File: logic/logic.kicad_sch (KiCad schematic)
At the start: 32 parts, among them J1 DIN41612_03x32_ABC, J2 Conn_02x05_Odd_Even, J3 Conn_02x05_Odd_Even, J5 Conn_02x02_Odd_Even, U1 TPIC6595, U11 LM7805_TO220, U2 TPIC6595, U3 TPIC6595, U4 TPIC6595, U5 TPIC6595, U6 TPIC6595, U7 TPIC6595, U8 TPIC6595, U9 74HC14

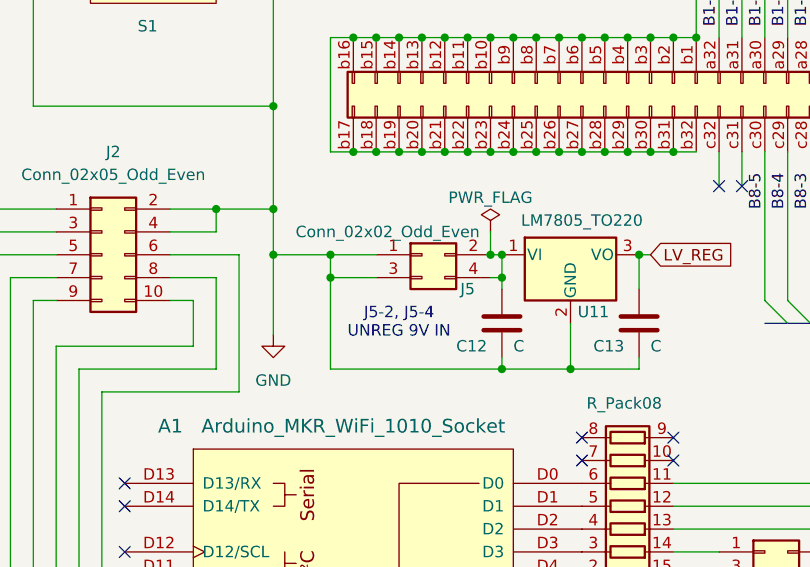
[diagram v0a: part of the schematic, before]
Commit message: Commit older work
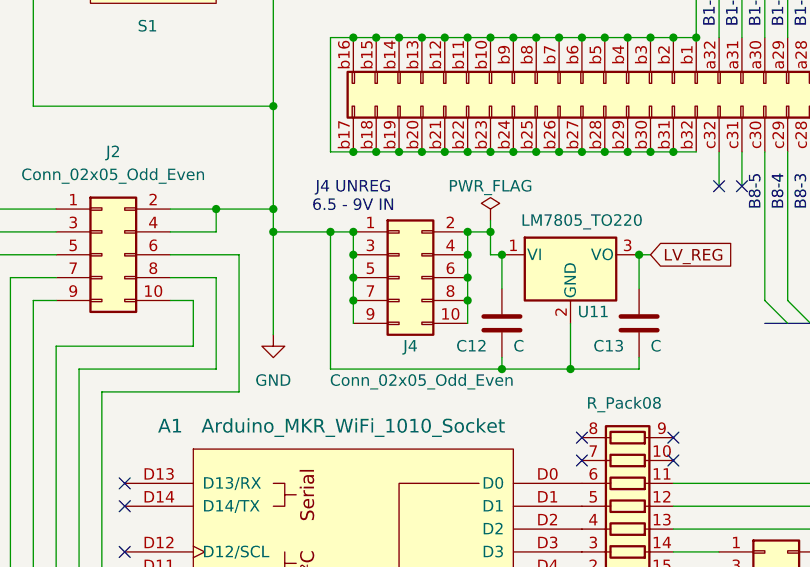
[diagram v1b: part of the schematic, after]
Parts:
- removed J5: Conn_02x02_Odd_Even, symbol Connector_Generic:Conn_02x02_Odd_Even
- added J4: Conn_02x05_Odd_Even, Connector_PinHeader_2.54mm:PinHeader_2x05_P2.54mm_Vertical, symbol Connector_Generic:Conn_02x05_Odd_Even
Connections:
- net GND: now also J4.1 (Pin_1), J4.3 (Pin_3), J4.5 (Pin_5), J4.7 (Pin_7), J4.9 (Pin_9)
- net at C12.1, U11.1 (VI): now also J4.10 (Pin_10), J4.2 (Pin_2), J4.4 (Pin_4), J4.6 (Pin_6), J4.8 (Pin_8)
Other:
- note added: "J4 UNREG 6.5 - 9V IN"
- note removed: "J5-2, J5-4 UNREG 9V IN"
